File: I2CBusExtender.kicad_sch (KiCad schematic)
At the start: 7 parts

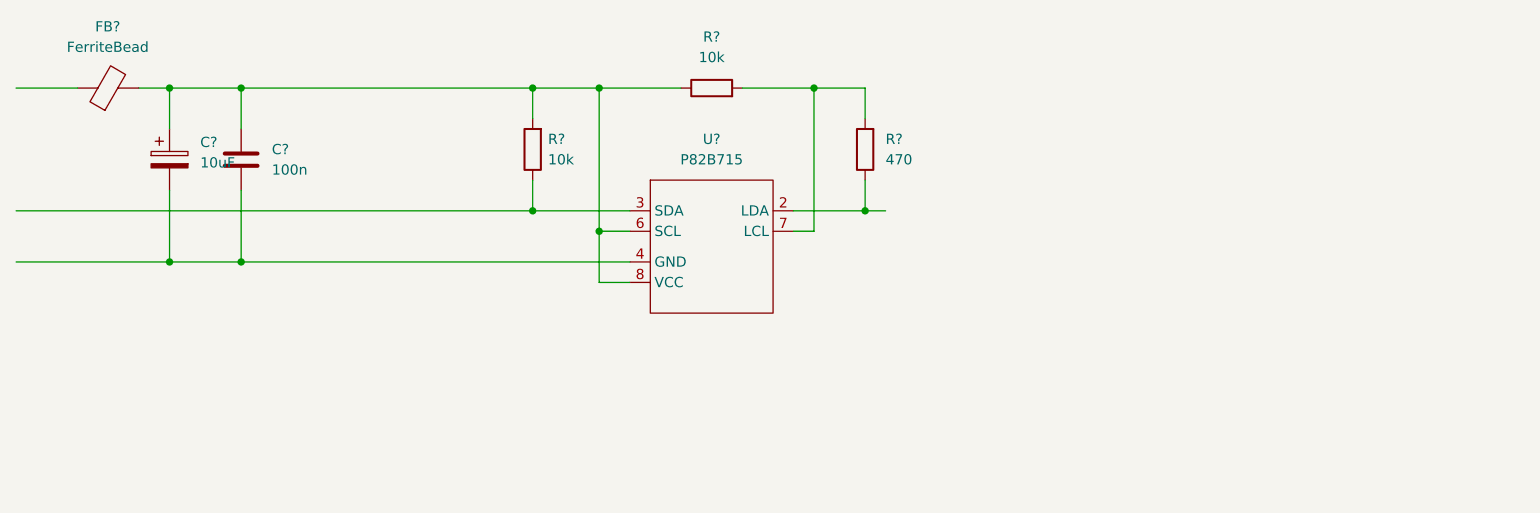
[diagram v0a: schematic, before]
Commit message: Initial schematic.
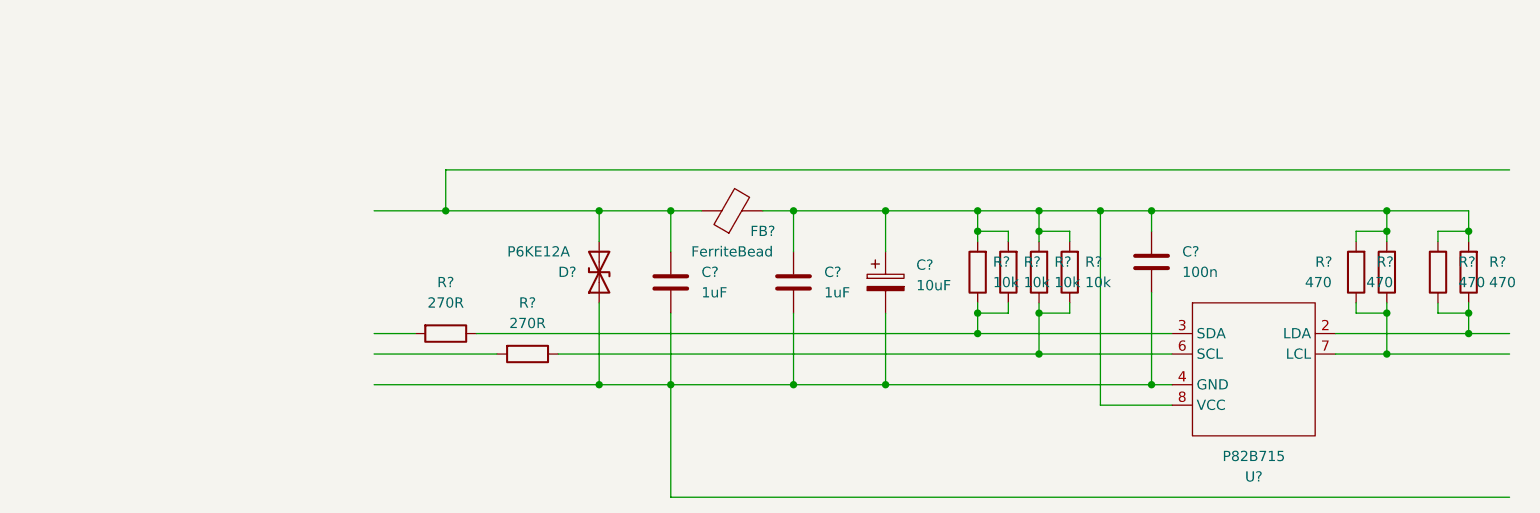
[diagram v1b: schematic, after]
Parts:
- removed R?: 10k, symbol Device:R
- added C? (x2): 1uF, symbol Device:C
- added D?: P6KE12A, symbol Device:D_TVS
- added R? (x2): 270R, symbol Device:R
- added R? (x3): 470, symbol Device:R
- added R? (x3): 10k, symbol Device:R
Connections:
- net at FB?.1: now also C?.1, D?.2 (A2)
- net at C?.1, C?.1, FB?.2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: now also R?.2, C?.1, R?.2, R?.2, R?.2, R?.2, R?.2, R?.2; no longer U?.6 (SCL)
- net at U?.7 (LCL): now also R?.1, R?.1; no longer R?.2
- net at R?.1, U?.2 (LDA): now also R?.1
- net at C?.2, C?.2, U?.4 (GND): now also C?.2, C?.2, D?.1 (A1)
- net at R?.1, U?.3 (SDA): now also R?.1, R?.1
- new net: R?.1, R?.1, R?.1, U?.6 (SCL)
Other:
- moved on the sheet: C?, FB?, R?, U?
